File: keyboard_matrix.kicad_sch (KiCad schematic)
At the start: 8 parts, among them SW2 A, SW3 S, SW4 D, SW5 W

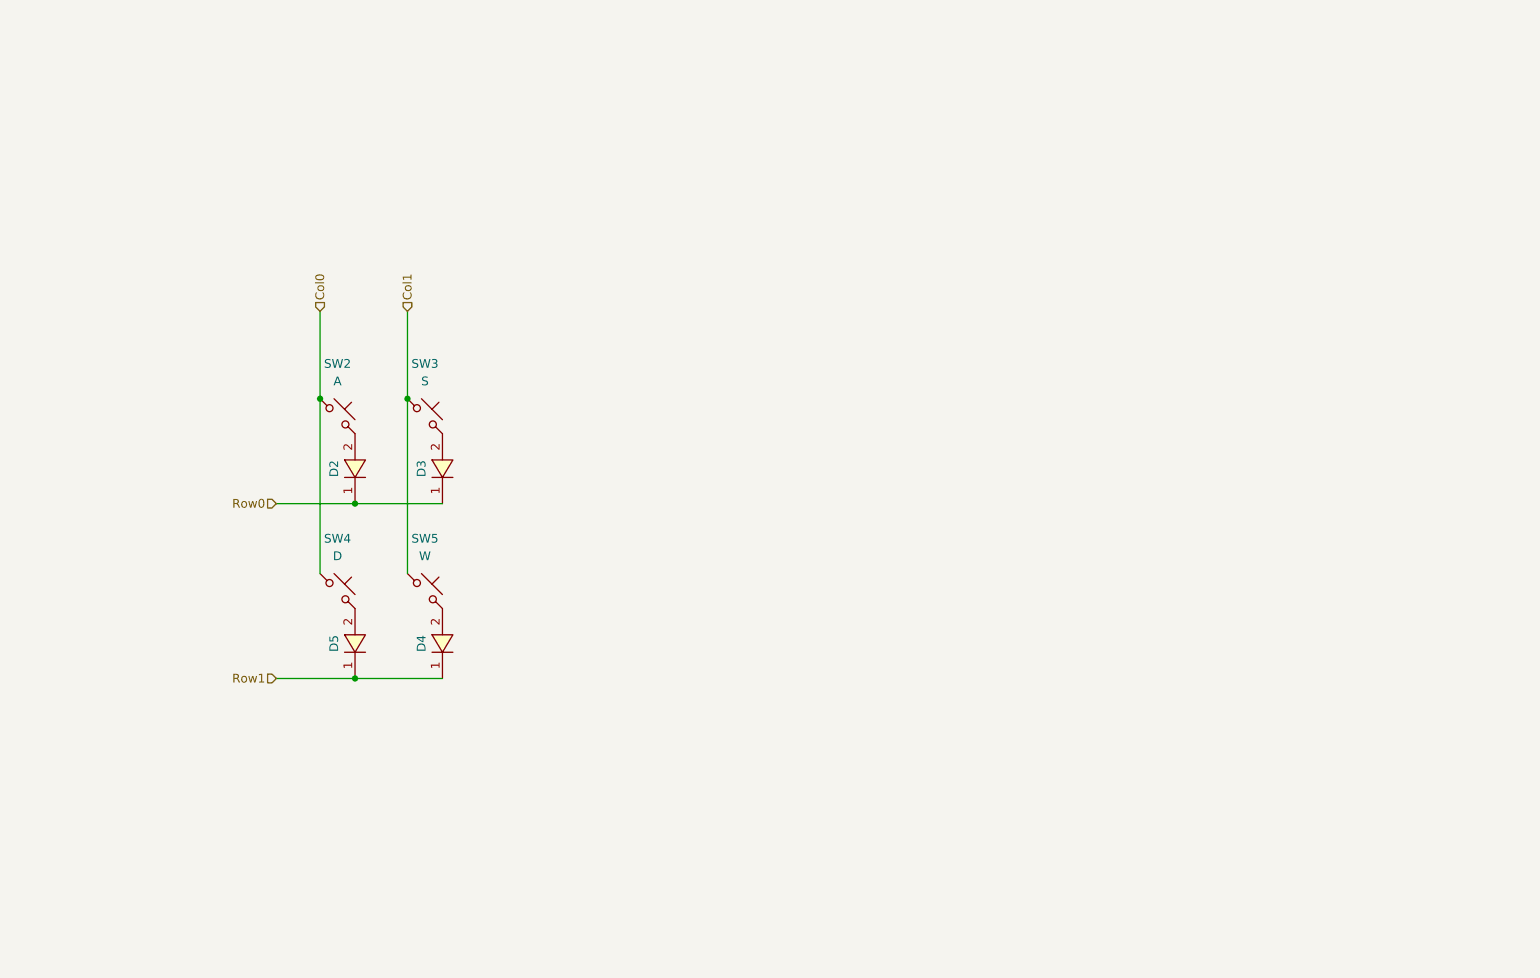
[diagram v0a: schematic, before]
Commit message: Update Migouner2.kicad_pcb, Migouner2.kicad_prl, Migouner2.kicad_pro, and 4 more files
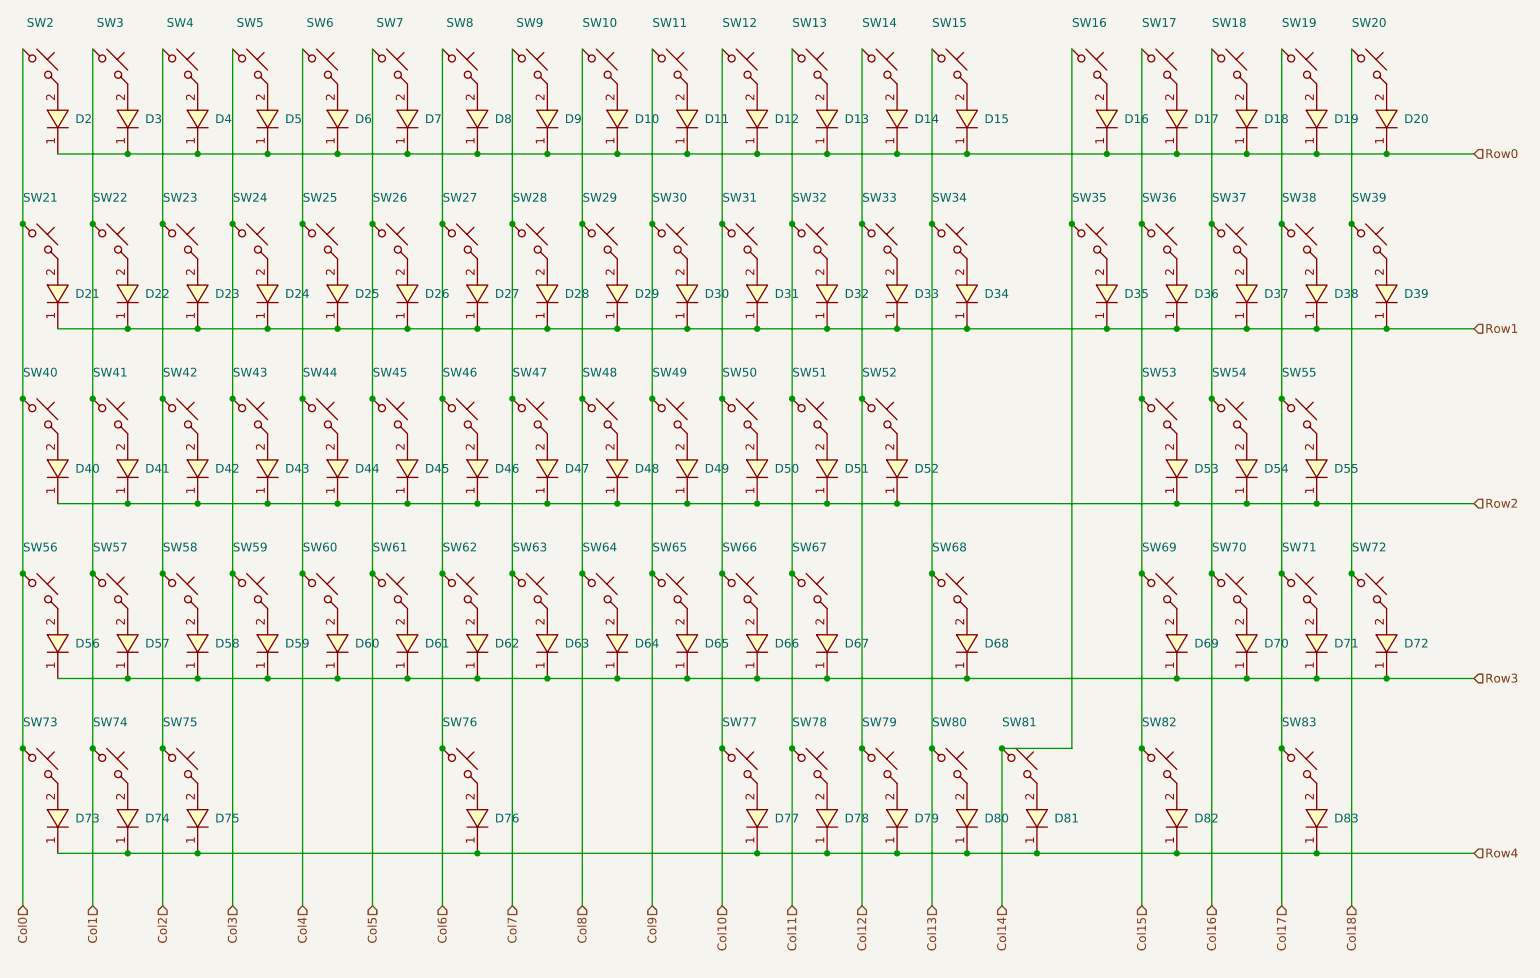
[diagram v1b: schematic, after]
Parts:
- added D10, D11, D12, D13, D14, D15, D16, D17, D18, D19, D20, D21, D23, D24, D25, D26, D27, D28, D29, D30, D31, D32, D33, D34, D35, D36, D37, D38, D39, D40, D42, D43, D44, D45, D46, D47, D48, D49, D50, D51, D52, D53, D54, D55, D56, D58, D59, D6, D60, D61, D62, D63, D64, D65, D66, D67, D68, D69, D7, D70, D71, D72, D73, D75, D76, D77, D78, D79, D8, D80, D81, D82, D83, D9: A, JLClib:SOD-323_L1.8-W1.3-LS2.5-RD, symbol JLClib:1N4148WST4
- added D22, D41, D57, D74: S, JLClib:SOD-323_L1.8-W1.3-LS2.5-RD, symbol JLClib:1N4148WST4
- added SW10, SW11, SW12, SW13, SW14, SW15, SW16, SW17, SW18, SW19, SW20, SW21, SW22, SW23, SW24, SW25, SW26, SW27, SW28, SW29, SW30, SW31, SW32, SW33, SW34, SW35, SW36, SW37, SW38, SW39, SW40, SW41, SW42, SW43, SW44, SW45, SW46, SW47, SW48, SW49, SW50, SW51, SW52, SW53, SW54, SW55, SW56, SW57, SW58, SW59, SW6, SW60, SW61, SW62, SW63, SW64, SW65, SW66, SW67, SW68, SW69, SW7, SW70, SW71, SW72, SW73, SW74, SW75, SW76, SW77, SW78, SW79, SW8, SW80, SW81, SW82, SW83, SW9: ~, JLClib:SW_Cherry_MX_1.00u_Plate, symbol Switch:SW_Push_45deg
- D4: value W -> A
- D5: value D -> A
- SW2: value A -> ~
- SW3: value S -> ~
- SW4: value D -> ~
- SW5: value W -> ~
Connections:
- net Col0: now also SW21.1, SW40.1, SW56.1, SW73.1; no longer SW4.1
- net Col1: now also SW22.1, SW41.1, SW57.1, SW74.1; no longer SW5.1
- net Row0: now also D4.1, D5.1, D10.1, D11.1, D12.1, D13.1, D14.1, D15.1, D16.1, D17.1, D18.1, D19.1, D20.1, D6.1, D7.1, D8.1, D9.1
- net Row1: now also D21.1, D22.1, D23.1, D24.1, D25.1, D26.1, D27.1, D28.1, D29.1, D30.1, D31.1, D32.1, D33.1, D34.1, D35.1, D36.1, D37.1, D38.1, D39.1; no longer D4.1, D5.1
- net at SW5.2: now also D5.2; no longer D4.2
- net at SW4.2: now also D4.2; no longer D5.2
- new net: D59.2, SW59.2
- new net: D52.2, SW52.2
- new net: D64.2, SW64.2
- new net: D46.2, SW46.2
- new net: D27.2, SW27.2
- new net: D26.2, SW26.2
- new net: D44.2, SW44.2
- new net: D60.2, SW60.2
- new net: D49.2, SW49.2
- new net: D81.2, SW81.2
- new net: D55.2, SW55.2
- new net: D67.2, SW67.2
- new net: D25.2, SW25.2
- new net: D14.2, SW14.2
- new net: D53.2, SW53.2
- new net: D77.2, SW77.2
- new net: D51.2, SW51.2
- new net: D13.2, SW13.2
- new net: D76.2, SW76.2
- new net: D43.2, SW43.2
- new net: D38.2, SW38.2
- new net: D83.2, SW83.2
- new net: D21.2, SW21.2
- new net: D63.2, SW63.2
- new net: D68.2, SW68.2
- new net: D65.2, SW65.2
- new net: D9.2, SW9.2
- new net: D74.2, SW74.2
- new net: D35.2, SW35.2
- new net: D15.2, SW15.2
- new net: D78.2, SW78.2
- new net: D58.2, SW58.2
- new net: D75.2, SW75.2
- new net: D12.2, SW12.2
- new net: D50.2, SW50.2
- new net: D24.2, SW24.2
- new net: D66.2, SW66.2
- new net: D28.2, SW28.2
- new net: D39.2, SW39.2
- new net: D57.2, SW57.2
- new net: D7.2, SW7.2
- new net: D16.2, SW16.2
- new net: D22.2, SW22.2
- new net: D62.2, SW62.2
- new net: D36.2, SW36.2
- new net: D69.2, SW69.2
- new net: D19.2, SW19.2
- new net: D29.2, SW29.2
- new net: D54.2, SW54.2
- new net: D72.2, SW72.2
- new net: D41.2, SW41.2
- new net: D34.2, SW34.2
- new net: D17.2, SW17.2
- new net: D80.2, SW80.2
- new net: D47.2, SW47.2
- new net: D30.2, SW30.2
- new net: D70.2, SW70.2
- new net: D56.2, SW56.2
- new net: D23.2, SW23.2
- new net: D8.2, SW8.2
- new net: D42.2, SW42.2
- new net: D31.2, SW31.2
- new net: D10.2, SW10.2
- new net: D82.2, SW82.2
- new net: D73.2, SW73.2
- new net: D48.2, SW48.2
- new net: D32.2, SW32.2
- new net: D33.2, SW33.2
- new net: D20.2, SW20.2
- new net: D71.2, SW71.2
- new net: D6.2, SW6.2
- new net: D18.2, SW18.2
- new net: D40.2, SW40.2
- new net: D61.2, SW61.2
- new net: D11.2, SW11.2
- new net: D45.2, SW45.2
- new net: D37.2, SW37.2
- new net: D79.2, SW79.2
- new net Col10: SW12.1, SW31.1, SW50.1, SW66.1, SW77.1
- new net Col11: SW13.1, SW32.1, SW51.1, SW67.1, SW78.1
- new net Col12: SW14.1, SW33.1, SW52.1, SW79.1
- new net Col13: SW15.1, SW34.1, SW68.1, SW80.1
- new net Col14: SW16.1, SW35.1, SW81.1
- new net Col15: SW17.1, SW36.1, SW53.1, SW69.1, SW82.1
- new net Col16: SW18.1, SW37.1, SW54.1, SW70.1
- new net Col17: SW19.1, SW38.1, SW55.1, SW71.1, SW83.1
- new net Col18: SW20.1, SW39.1, SW72.1
- new net Col2: SW23.1, SW4.1, SW42.1, SW58.1, SW75.1
- new net Col3: SW24.1, SW43.1, SW5.1, SW59.1
- new net Col4: SW25.1, SW44.1, SW6.1, SW60.1
- new net Col5: SW26.1, SW45.1, SW61.1, SW7.1
- new net Col6: SW27.1, SW46.1, SW62.1, SW76.1, SW8.1
- new net Col7: SW28.1, SW47.1, SW63.1, SW9.1
- new net Col8: SW10.1, SW29.1, SW48.1, SW64.1
- new net Col9: SW11.1, SW30.1, SW49.1, SW65.1
- new net Row2: D40.1, D41.1, D42.1, D43.1, D44.1, D45.1, D46.1, D47.1, D48.1, D49.1, D50.1, D51.1, D52.1, D53.1, D54.1, D55.1
- new net Row3: D56.1, D57.1, D58.1, D59.1, D60.1, D61.1, D62.1, D63.1, D64.1, D65.1, D66.1, D67.1, D68.1, D69.1, D70.1, D71.1, D72.1
- new net Row4: D73.1, D74.1, D75.1, D76.1, D77.1, D78.1, D79.1, D80.1, D81.1, D82.1, D83.1
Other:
- moved on the sheet: D2, D3, SW2, SW3
